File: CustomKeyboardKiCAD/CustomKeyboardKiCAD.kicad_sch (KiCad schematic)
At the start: 56 parts, among them J1 USB_C_Receptacle_USB2.0_16P, J3 S2B-PH-K-SLFSN, SW91 RotaryEncoder_Switch, U1 nRF52840, U2 XC6220B331MR, U3 74HC595, U4 BQ24075RGTR, U5 74HC595, U6 74HC595, U7 nice_nano, Y1 32.768kHz FC-12M, Y2 32MHz XRCGB32MOODF1H5ORO

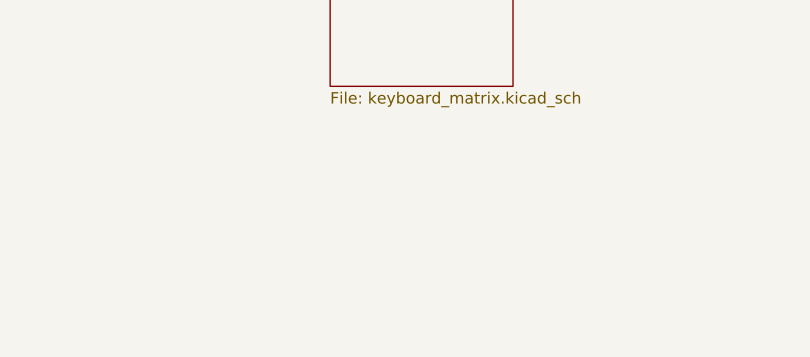
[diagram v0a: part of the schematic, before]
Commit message: schematic is generally complete
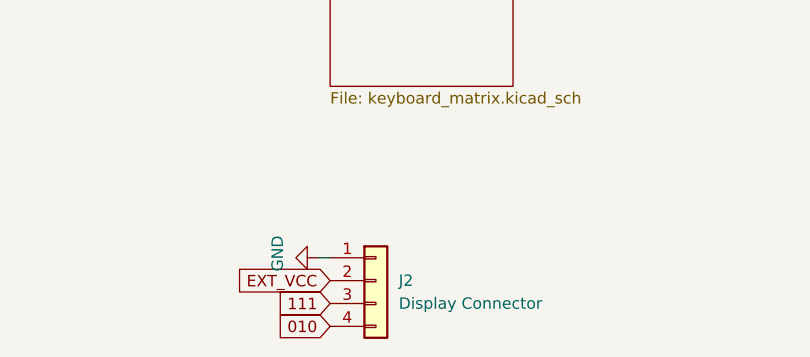
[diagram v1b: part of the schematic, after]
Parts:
- added J2: Display Connector, Connector_PinHeader_2.54mm:PinHeader_1x04_P2.54mm_Vertical, symbol Connector_Generic:Conn_01x04
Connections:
- net 010: now also J2.4 (Pin_4)
- net 111: now also J2.3 (Pin_3)
- net EXT_VCC: now also J2.2 (Pin_2)
- net GND: now also J2.1 (Pin_1)
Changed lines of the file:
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@@
 	(wire
 		(pts
+			(xy 212.09 290.83) (xy 213.36 290.83)
+		)
+		(stroke
+			(width 0)
+			(type default)
+		)
+	)
+	(wire
+		(pts
 			(xy 281.94 80.01) (xy 281.94 83.82)
 		)
@@
 		)
 	)
+	(global_label "010"
+		(shape input)
+		(at 213.36 298.45 180)
+		(fields_autoplaced yes)
+		(effects
+			(font
+				(size 1.27 1.27)
+			)
+			(justify right)
+		)
+		(property "Intersheetrefs" "${INTERSHEET_REFS}"
+			(at 206.7463 298.45 0)
+			(effects
+				(font
+					(size 1.27 1.27)
+				)
+				(justify right)
+				(hide yes)
+			)
+		)
+	)
 	(global_label "113"
 		(shape input)
@@
 		)
 	)
+	(global_label "EXT_VCC"
+		(shape input)
+		(at 213.36 293.37 180)
+		(fields_autoplaced yes)
+		(effects
+			(font
+				(size 1.27 1.27)
+			)
+			(justify right)
+		)
+		(property "Intersheetrefs" "${INTERSHEET_REFS}"
+			(at 202.4525 293.37 0)
+			(effects
+				(font
+					(size 1.27 1.27)
+				)
+				(justify right)
+				(hide yes)
+			)
+		)
+	)
 	(global_label "008"
 		(shape input)
@@
 		)
 	)
+	(global_label "111"
+		(shape input)
+		(at 213.36 295.91 180)
+		(fields_autoplaced yes)
+		(effects
+			(font
+				(size 1.27 1.27)
+			)
+			(justify right)
+		)
+		(property "Intersheetrefs" "${INTERSHEET_REFS}"
+			(at 206.7463 295.91 0)
+			(effects
+				(font
+					(size 1.27 1.27)
+				)
+				(justify right)
+				(hide yes)
+			)
+		)
+	)
 	(global_label "BLED"
 		(shape input)
@@
 	)
 	(symbol
+		(lib_id "Connector_Generic:Conn_01x04")
+		(at 218.44 293.37 0)
+		(unit 1)
+		(exclude_from_sim no)
+		(in_bom yes)
+		(on_board yes)
+		(dnp no)
+		(fields_autoplaced yes)
+		(property "Reference" "J2"
+			(at 220.98 293.3699 0)
+			(effects
+				(font
+					(size 1.27 1.27)
+				)
+				(justify left)
+			)
+		)
+		(property "Value" "Display Connector"
+			(at 220.98 295.9099 0)
+			(effects
+				(font
+					(size 1.27 1.27)
+				)
+				(justify left)
+			)
+		)
+		(property "Footprint" "Connector_PinHeader_2.54mm:PinHeader_1x04_P2.54mm_Vertical"
+			(at 218.44 293.37 0)
+			(effects
+				(font
+					(size 1.27 1.27)
+				)
+				(hide yes)
+			)
+		)
+		(property "Datasheet" "~"
+			(at 218.44 293.37 0)
+			(effects
+				(font
+					(size 1.27 1.27)
+				)
+				(hide yes)
+			)
+		)
+		(property "Description" "Generic connector, single row, 01x04, script generated (kicad-library-utils/schlib/autogen/connector/)"
+			(at 218.44 293.37 0)
+			(effects
+				(font
+					(size 1.27 1.27)
+				)
+				(hide yes)
+			)
+		)
+		(pin "1"
+		)
+		(pin "2"
+		)
+		(pin "4"
+		)
+		(pin "3"
+		)
+		(instances
+			(project ""
+				(path "/aaa1400c-18c9-4b83-ab7e-c530ca104a6d"
+					(reference "J2")
+					(unit 1)
+				)
+			)
+		)
+	)
+	(symbol
 		(lib_id "power:GND")
 		(at 39.37 153.67 0)
@@
 					(unit 1)
 				)
+			)
+		)
+	)
+	(symbol
+		(lib_id "power:GND")
+		(at 212.09 290.83 270)
+		(unit 1)
+		(exclude_from_sim no)
+		(in_bom yes)
+		(on_board yes)
+		(dnp no)
+		(property "Reference" "#PWR053"
+			(at 205.74 290.83 0)
+			(effects
+				(font
+					(size 1.27 1.27)
+				)
+				(hide yes)
+			)
+		)
+		(property "Value" "GND"
+			(at 207.518 292.354 0)
+			(effects
+				(font
+					(size 1.27 1.27)
+				)
+				(justify right)
+			)
+		)
+		(property "Footprint" ""
+			(at 212.09 290.83 0)
+			(effects
+				(font
+					(size 1.27 1.27)
+				)
+				(hide yes)
+			)
+		)
+		(property "Datasheet" ""
+			(at 212.09 290.83 0)
+			(effects
+				(font
+					(size 1.27 1.27)
+				)
+				(hide yes)
+			)
+		)
+		(property "Description" "Power symbol creates a global label with name \"GND\" , ground"
+			(at 212.09 290.83 0)
+			(effects
+				(font
+					(size 1.27 1.27)
+				)
+				(hide yes)
+			)
+		)
+		(pin "1"
+		)
+		(instances
+			(project "CustomKeyboardKiCAD"
+				(path "/aaa1400c-18c9-4b83-ab7e-c530ca104a6d"
+					(reference "#PWR053")
+					(unit 1)
+				)
